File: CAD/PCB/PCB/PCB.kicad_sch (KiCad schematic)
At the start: 10 parts, among them J1 Screw_Terminal_01x02, J2 Conn_01x06_Socket, J3 Conn_01x04_Socket, J4 Conn_01x06_Socket, J5 Screw_Terminal_01x04, J6 Conn_01x04_Socket, U1 PC817, U2 WeAct-RP2040-Pico

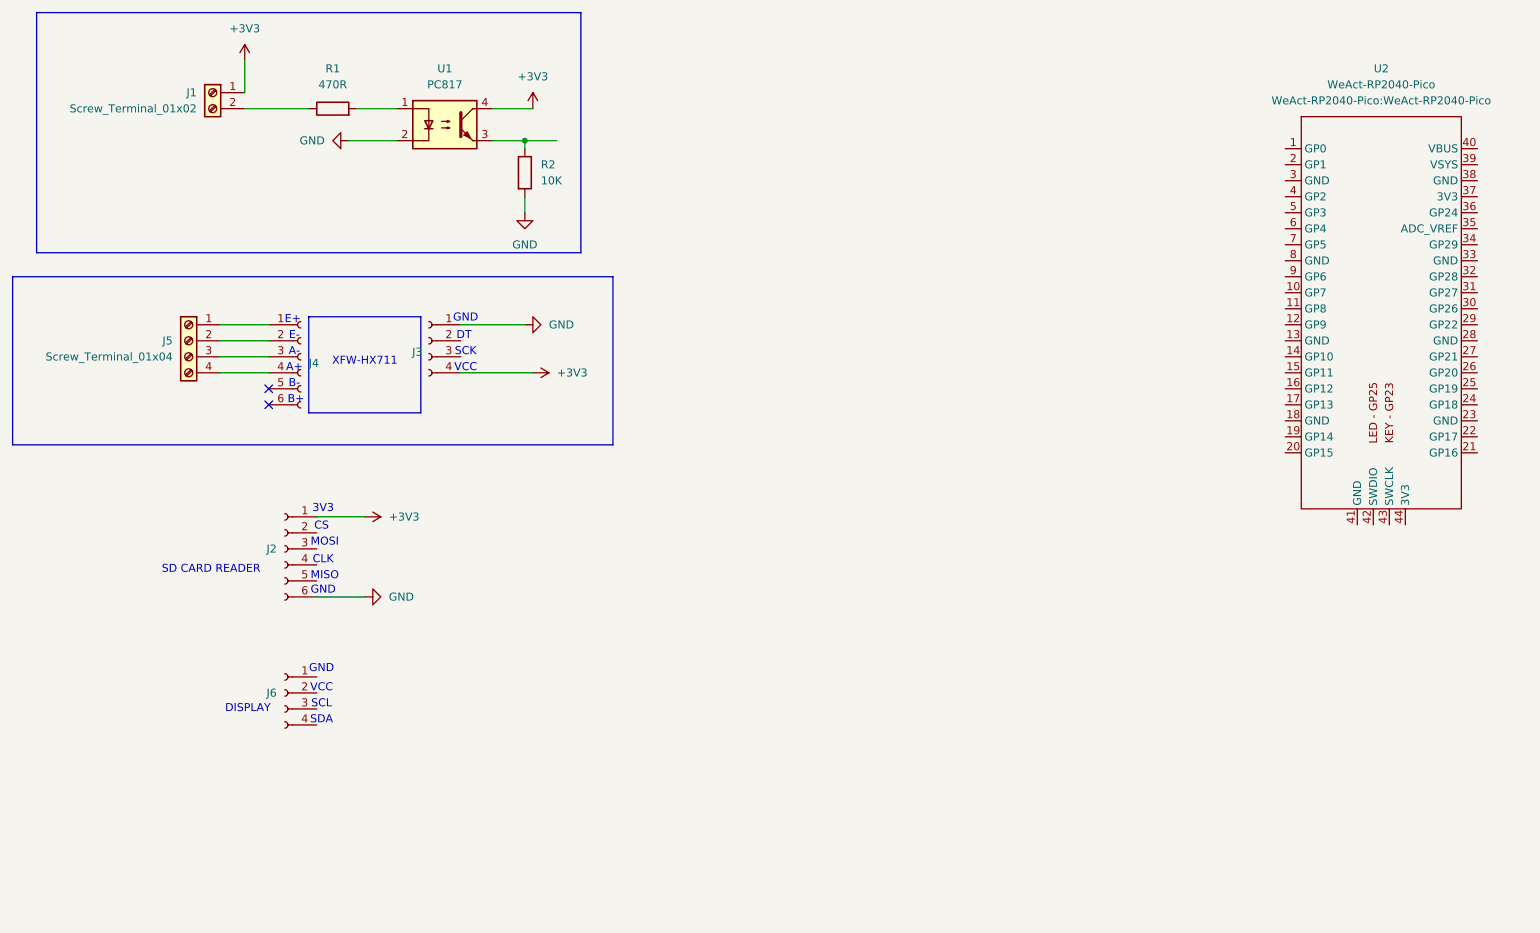
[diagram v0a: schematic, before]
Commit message: CAD
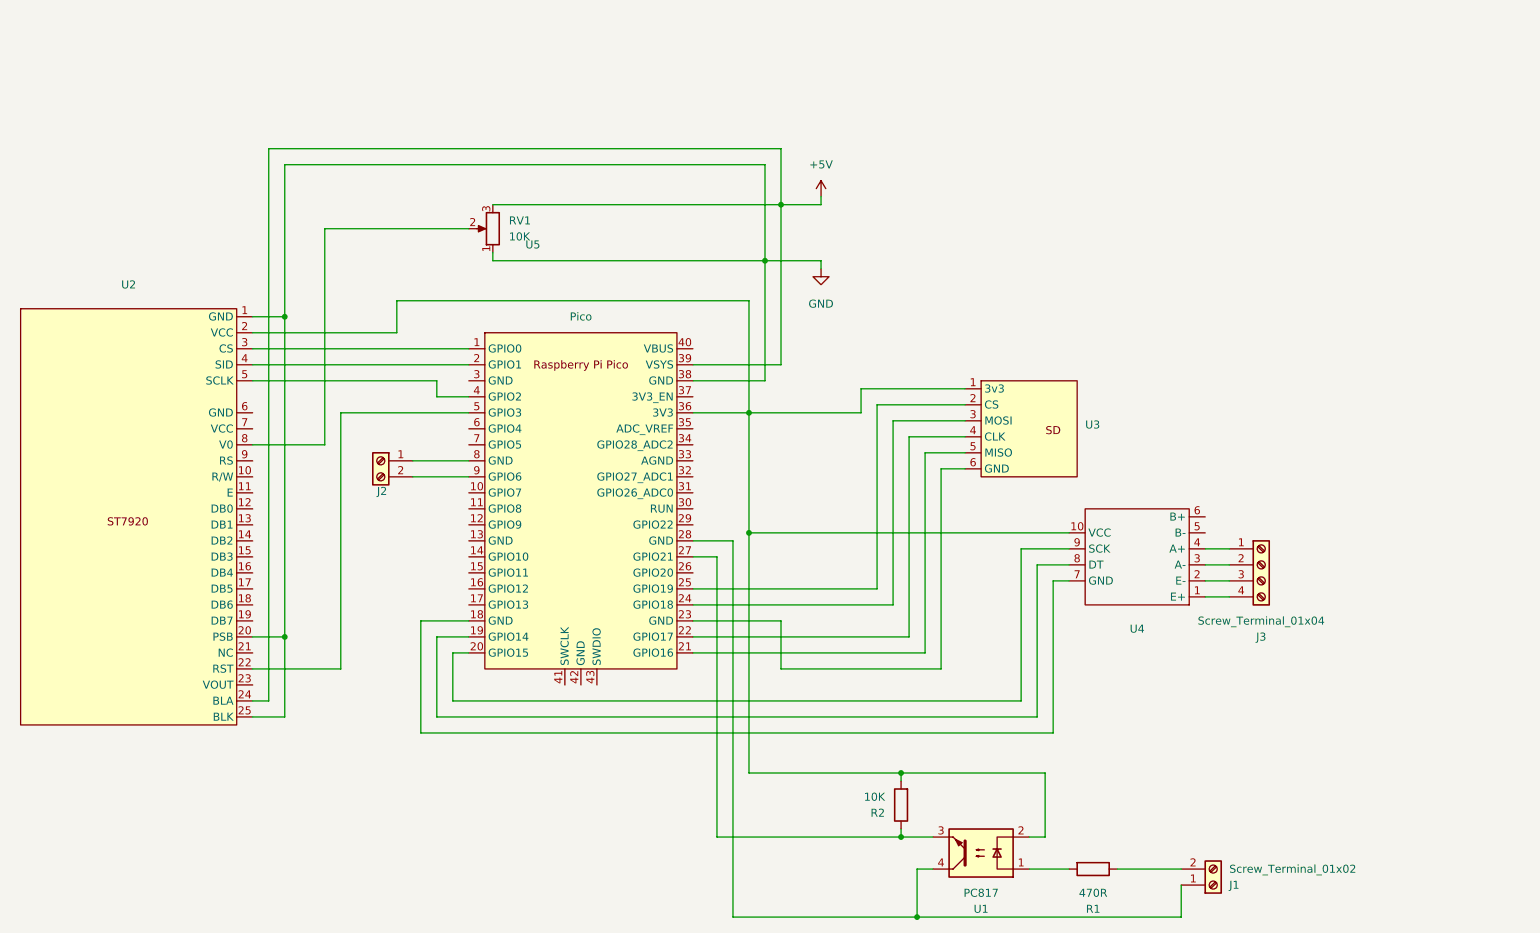
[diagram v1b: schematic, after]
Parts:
- removed J2: Conn_01x06_Socket, symbol Connector:Conn_01x06_Socket
- removed J3, J6: Conn_01x04_Socket, symbol Connector:Conn_01x04_Socket
- removed J4: Conn_01x06_Socket, Connector_PinSocket_1.00mm:PinSocket_1x06_P1.00mm_Vertical, symbol Connector:Conn_01x06_Socket
- removed J5: Screw_Terminal_01x04, symbol Connector:Screw_Terminal_01x04
- removed U2: WeAct-RP2040-Pico, WeAct-RP2040-Pico:WeAct-RP2040-Pico, symbol WeAct-RP2040-Pico:WeAct-RP2040-Pico
- added J2: Screw_Terminal_01x02, symbol Connector:Screw_Terminal_01x02
- added J3: Screw_Terminal_01x04, TerminalBlock:TerminalBlock_Altech_AK300-4_P5.00mm, symbol Connector:Screw_Terminal_01x04
- added RV1: 10K, symbol Device:R_Potentiometer
- added U2: ~, symbol New_Library:ST7920
- added U3: ~, symbol New_Library:MicroSD_reader
- added U4: ~, symbol New_Library:XFW-HX711
- added U5: Pico, RPi_Pico:RPi_Pico_SMD_TH, symbol MCU_RaspberryPi_and_Boards:Pico
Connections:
- net GND: now also RV1.1, U2.1 (GND), U2.20 (PSB), U2.25 (BLK), U5.38 (GND); no longer R2.2, U1.2
- net at R2.1, U1.3: now also U5.27 (GPIO21)
- net +3V3: no longer names the net of J1.1 (Pin_1), U1.4
- net +3V3: now also U5.28 (GND)
- new net: R2.2, U1.2, U2.2 (VCC), U3.1 (3v3), U4.10 (VCC), U5.36 (3V3)
- new net: U2.22 (RST), U5.5 (GPIO3)
- new net: U2.3 (CS), U5.1 (GPIO0)
- new net: U2.4 (SID), U5.2 (GPIO1)
- new net: U2.5 (SCLK), U5.4 (GPIO2)
- new net: RV1.2, U2.8 (V0)
- new net: U3.2 (CS), U5.25 (GPIO19)
- new net: U3.3 (MOSI), U5.24 (GPIO18)
- new net: U3.4 (CLK), U5.22 (GPIO17)
- new net: U3.5 (MISO), U5.21 (GPIO16)
- new net: U3.6 (GND), U5.23 (GND)
- new net: U4.7 (GND), U5.18 (GND)
- new net: U4.8 (DT), U5.19 (GPIO14)
- new net: U4.9 (SCK), U5.20 (GPIO15)
- new net: J2.1 (Pin_1), U5.8 (GND)
- new net: J2.2 (Pin_2), U5.9 (GPIO6)
- new net: J3.4 (Pin_4), U4.1 (E+)
- new net: J3.3 (Pin_3), U4.2 (E-)
- new net: J3.2 (Pin_2), U4.3 (A-)
- new net: J3.1 (Pin_1), U4.4 (A+)
- new net +5V: RV1.3, U2.24 (BLA), U5.39 (VSYS)
- no-connect marks 2 -> 0
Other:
- note removed: "3V3"
- note removed: "A+"
- note removed: "A-"
- note removed: "B+"
- note removed: "B-"
- note removed: "CLK"
- note removed: "CS"
- note removed: "DISPLAY"
- note removed: "DT"
- note removed: "E+"
- note removed: "E-"
- note removed: "GND"
- note removed: "MISO"
- note removed: "MOSI"
- note removed: "SCK"
- note removed: "SCL"
- note removed: "SD CARD READER"
- note removed: "SDA"
- note removed: "VCC"
- note removed: "XFW-HX711"
- moved on the sheet: J1, R1, R2, U1
